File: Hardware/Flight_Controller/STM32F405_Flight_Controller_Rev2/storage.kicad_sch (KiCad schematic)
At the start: 2 parts, among them U5 W25Q128JVS

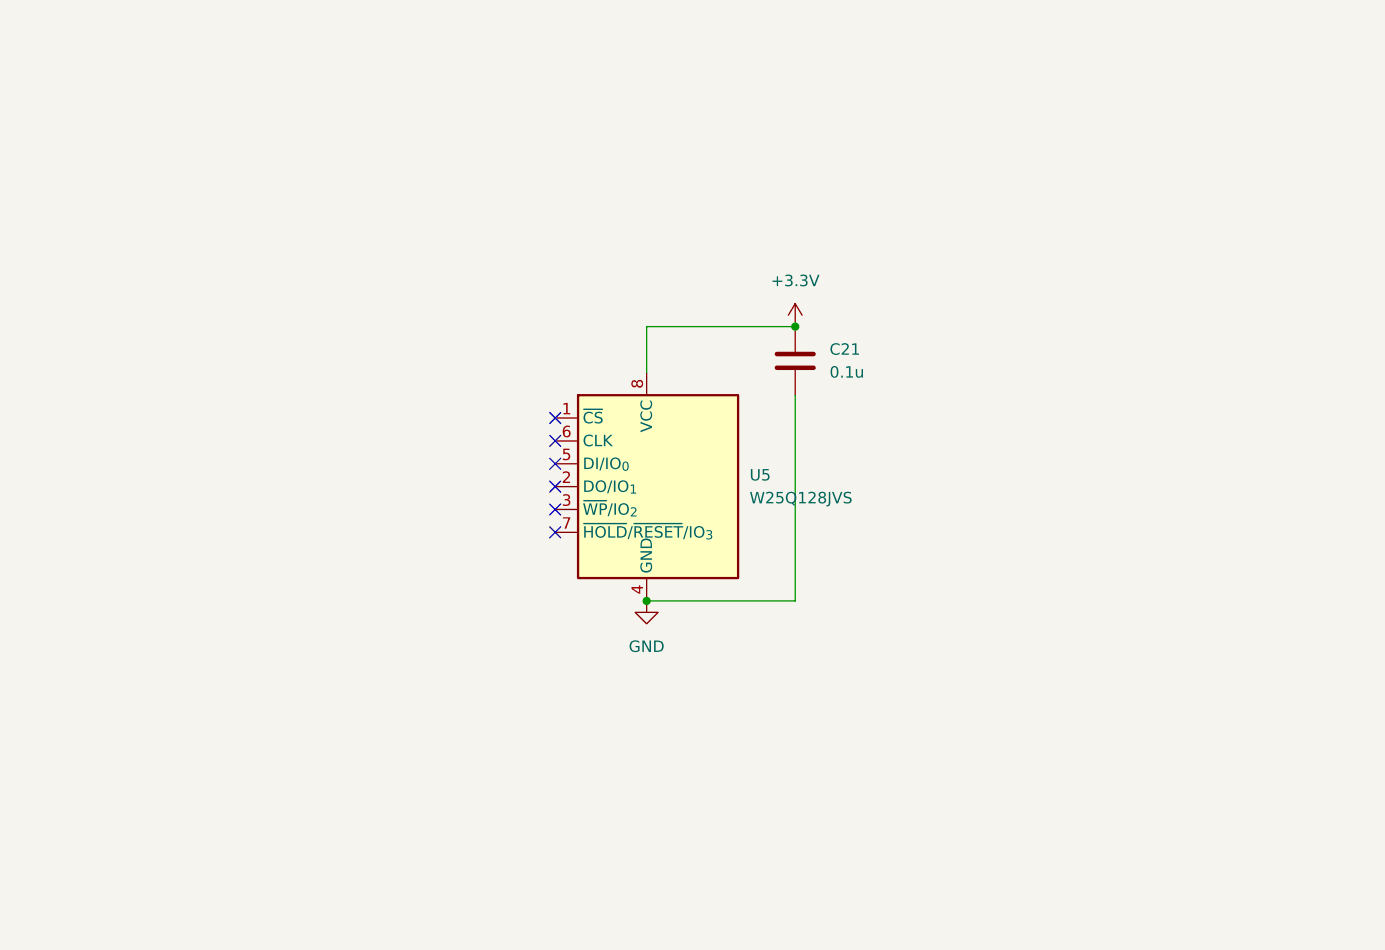
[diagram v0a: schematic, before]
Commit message: Ready Rev2 PCB
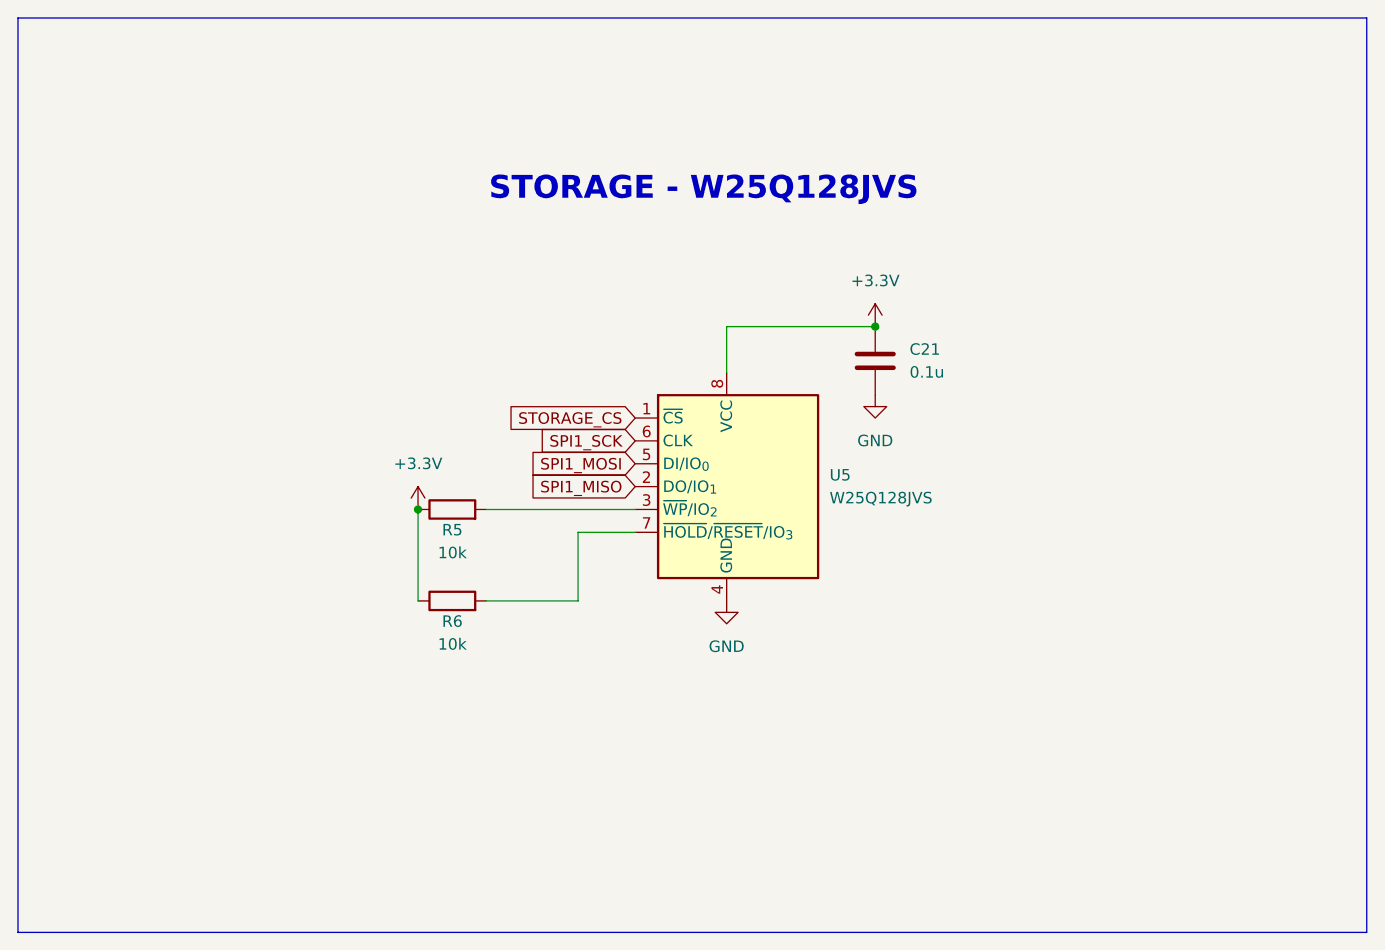
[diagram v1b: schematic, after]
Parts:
- added R5, R6: 10k, Resistor_SMD:R_0603_1608Metric_Pad0.98x0.95mm_HandSolder, symbol Device:R
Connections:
- net +3.3V: now also R5.1, R6.1
- net STORAGE_CS: now reaches U5.1 (~{CS})
- net SPI1_MISO: now reaches U5.2 (DO/IO_{1})
- net at U5.3 (~{WP}/IO_{2}): now also R5.2
- net SPI1_MOSI: now reaches U5.5 (DI/IO_{0})
- net SPI1_SCK: now reaches U5.6 (CLK)
- net at U5.7 (~{HOLD}/~{RESET}/IO_{3}): now also R6.2
- no-connect marks 6 -> 0
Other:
- note added: "STORAGE - W25Q128JVS"
- moved on the sheet: C21, U5
